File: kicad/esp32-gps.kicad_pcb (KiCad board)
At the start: 4 copper layers, 50 x 50 mm, 61 parts, among them J1 MHF4, J2 MHF4, P1 USB_C_Plug_USB2.0, Q1 BCW66G, Q2 BCW66G, Q3 Si2319CDS, SW1 RESET, SW2 BOOT, U1 ESP32-PICO-V3, U10 Battery, U11 AP2112K-3.3, U2 GP-01, U3 CP2102N-Axx-xQFN28, U4 TP4056-42-ESOP8, U5 USBLC6-2P6, U6 U8205A, U7 DW01A, U8 LTC4412, U9 Switch

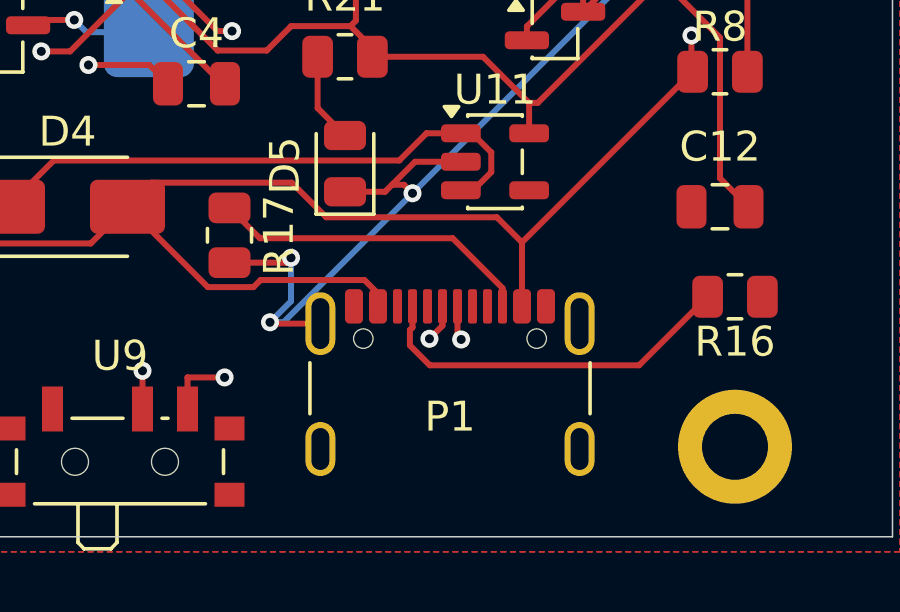
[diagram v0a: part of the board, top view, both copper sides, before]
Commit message: init
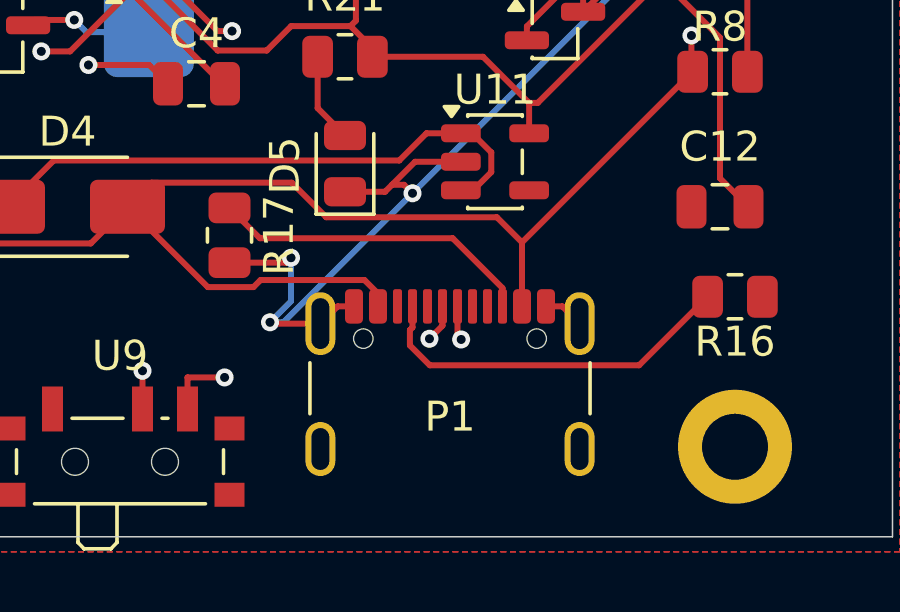
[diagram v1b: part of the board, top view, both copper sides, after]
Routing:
- net GND: track 153.0 -> 155.7 mm
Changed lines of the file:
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@@
+	)
+	(segment
+		(start 160.755 113.32)
+		(end 160.18 113.895)
+		(width 0.2)
+		(layer "F.Cu")
+		(net 1)
 	)
 	(segment
@@
 	)
 	(segment
+		(start 167.7 113.32)
+		(end 168.245 113.32)
+		(width 0.2)
+		(layer "F.Cu")
+		(net 1)
+	)
+	(segment
 		(start 154.5 82.9)
 		(end 154.95 83.35)
@@
 		(width 0.2)
 		(layer "F.Cu")
+		(net 1)
+	)
+	(segment
+		(start 161.3 113.32)
+		(end 160.755 113.32)
+		(width 0.2)
+		(layer "F.Cu")
+		(net 1)
+	)
+	(segment
+		(start 168.245 113.32)
+		(end 168.82 113.895)
+		(width 0.2)
+		(layer "F.Cu")
